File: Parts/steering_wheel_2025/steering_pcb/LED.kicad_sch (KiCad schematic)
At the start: 3 parts, among them J13 PINHD_1x1_Male, Q4 BS170

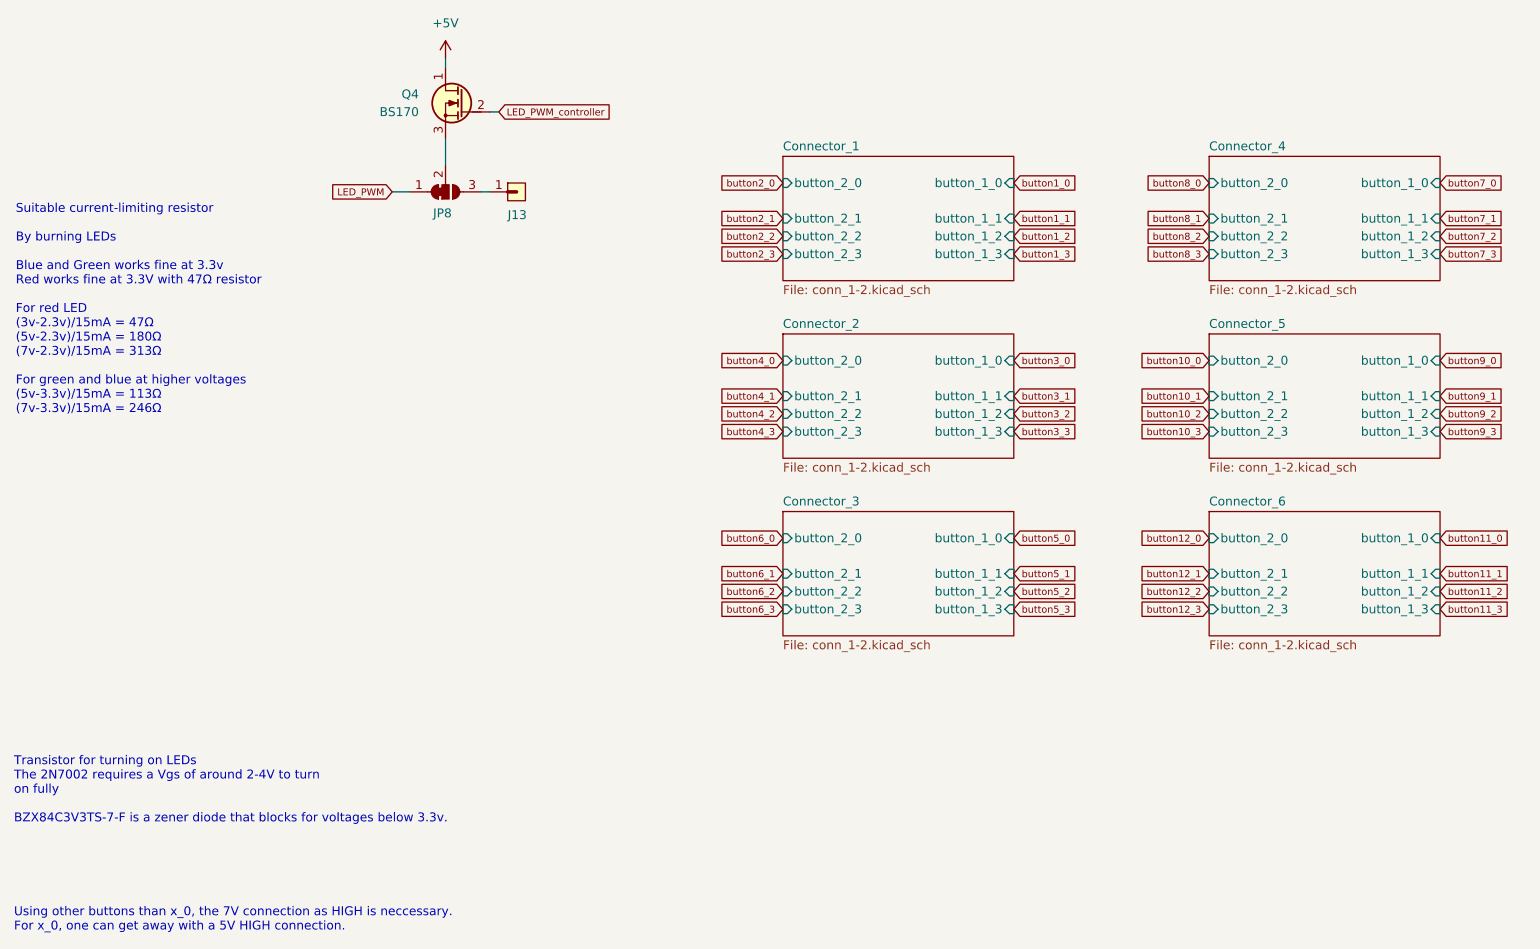
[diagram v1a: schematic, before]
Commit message: Dashboard electron
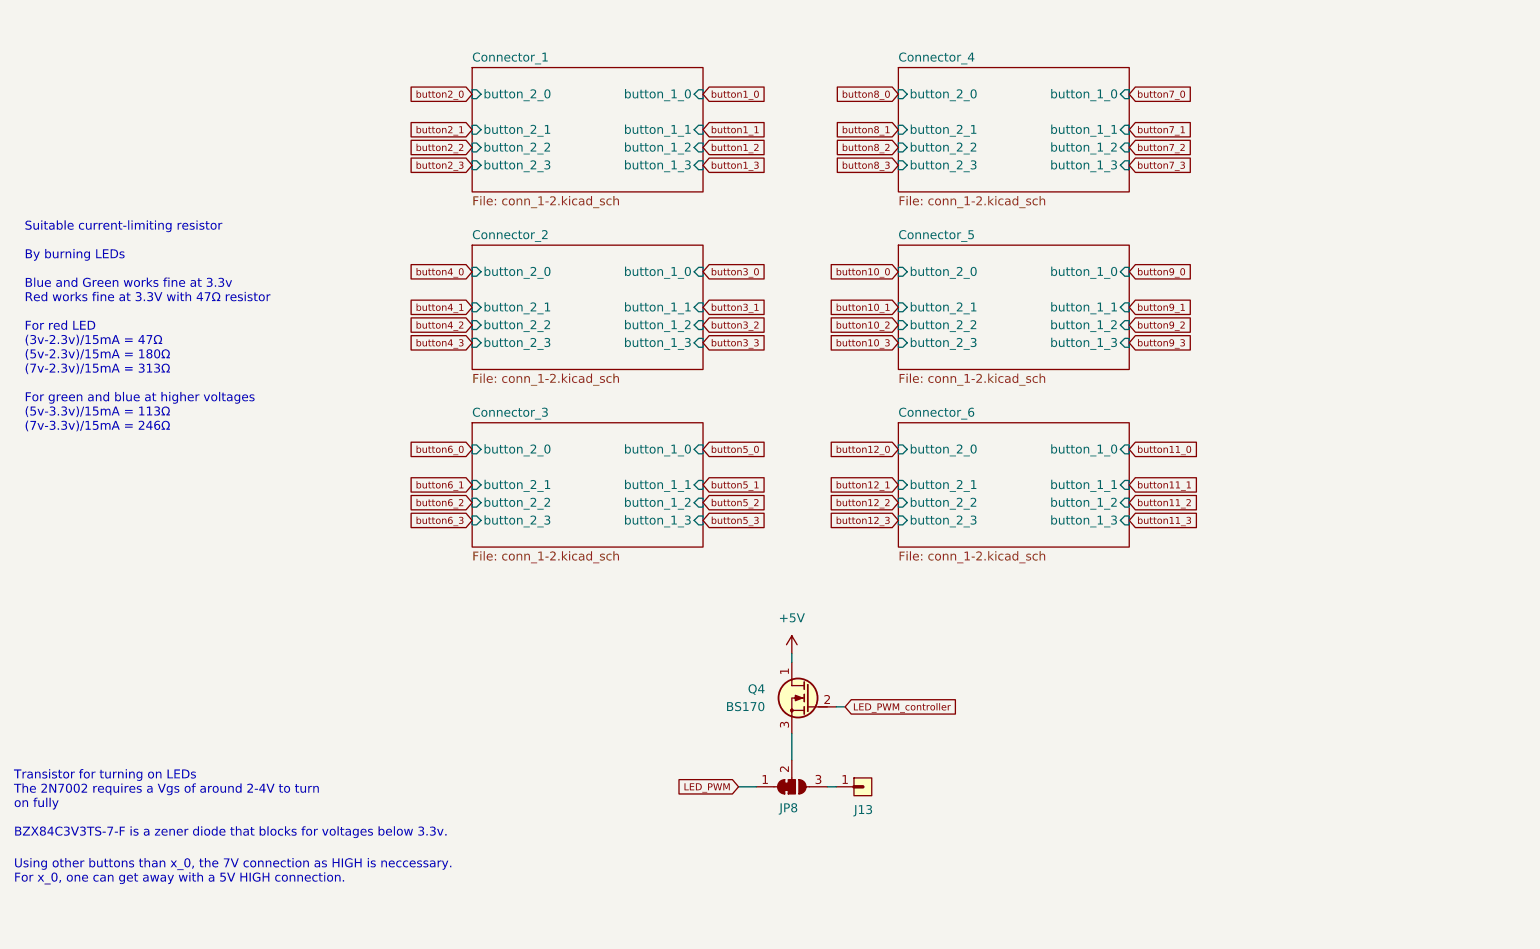
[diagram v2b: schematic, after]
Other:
- moved on the sheet: J13, JP8, Q4
